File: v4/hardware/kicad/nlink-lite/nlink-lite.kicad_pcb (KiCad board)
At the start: 4 copper layers, 39 x 16 mm, 21 parts, among them J1 USB_MiniB_PLUG_to_calc, J4 PROG_PADS_TC2030, SW1 PWR_SW, U1 ESP32-C3-MINI-1-N4, U3 CP2102N-A02-GQFN24, U4 TLV62569DBV, U5 USBLC6-2SC6

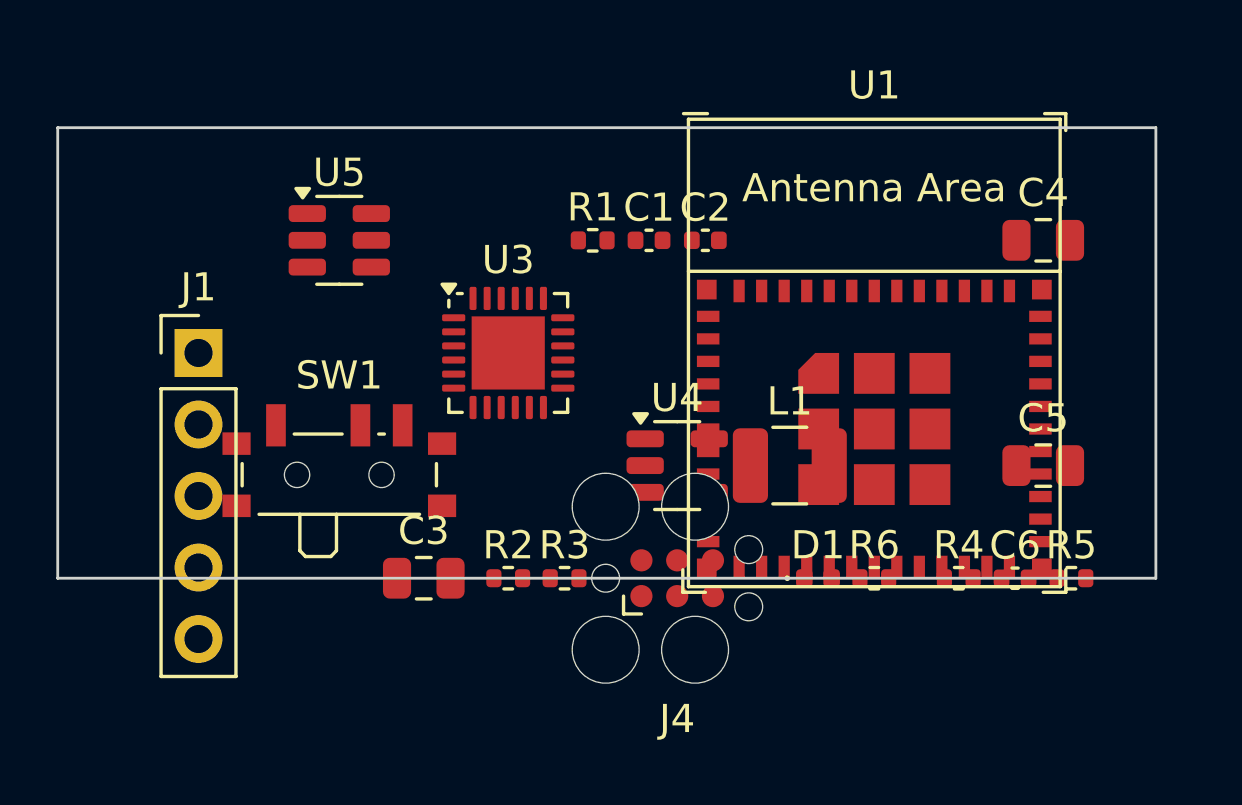
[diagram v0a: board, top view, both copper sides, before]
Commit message: Updated v4 pcb
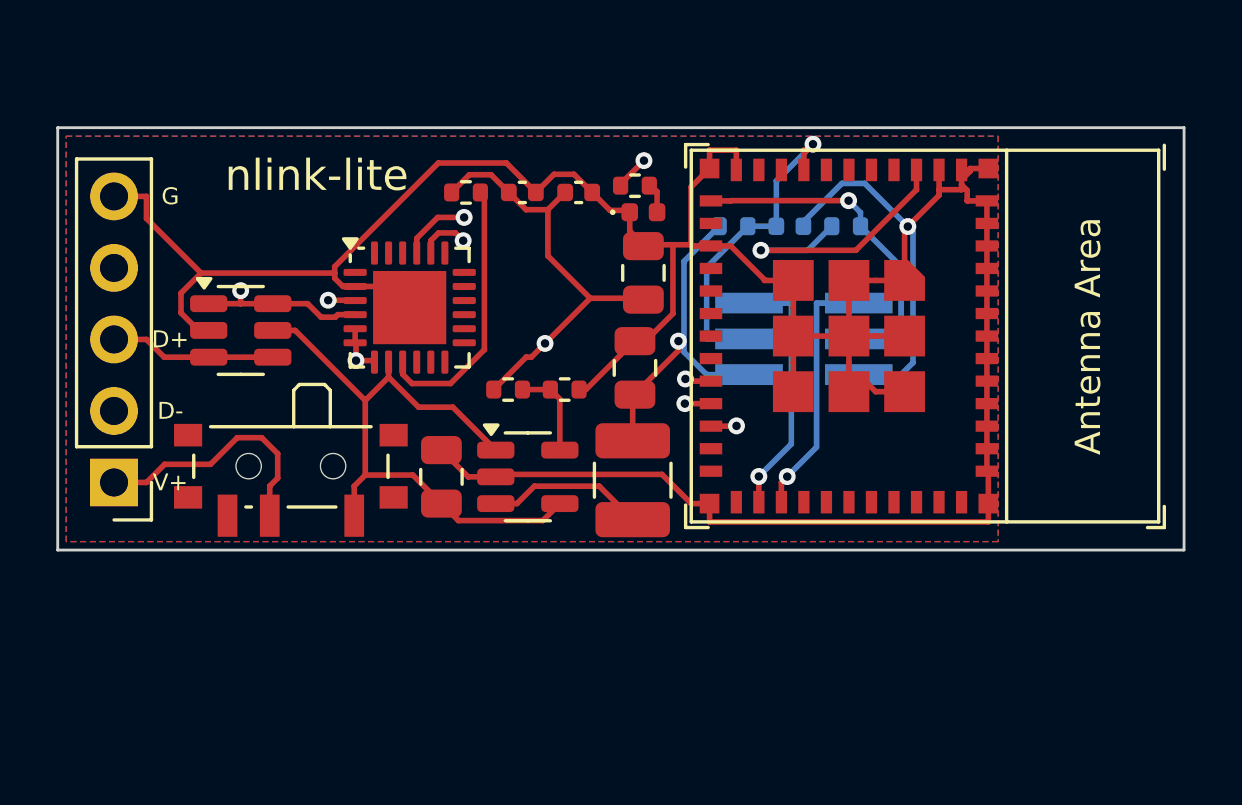
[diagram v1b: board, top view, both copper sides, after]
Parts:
- C6, R4, R5: moved to B.Cu
- J4: value PROG_PADS_TC2030 -> PROG_PADS_2x3_POGO; footprint Connector:Tag-Connect_TC2030-IDC-FP_2x03_P1.27mm_Vertical -> Connector_PinHeader_1.27mm:PinHeader_2x03_P1.27mm_Vertical_SMD; moved to B.Cu
- moved R6 16.3 mm to (70.5, 52.1)
- moved C5 15.8 mm to (70.8, 55.2), turned to 90 degrees
- moved C4 15.2 mm to (70.5, 58.5), turned to 90 degrees
- moved C6 14.8 mm to (76.0, 53.5)
- moved R4 14.8 mm to (74.0, 53.5)
- moved R5 14.8 mm to (78.0, 53.5)
- moved D1 14.4 mm to (70.8, 53.0)
- moved J4 9.62 mm to (76.5, 57.5)
- moved R2 6.70 mm to (66.0, 59.3)
- moved R3 6.70 mm to (68.0, 59.3)
- moved L1 5.60 mm to (70.4, 62.5), turned to 90 degrees
- moved J1 5.49 mm to (52.0, 62.6), turned to 180 degrees
- moved U4 5.32 mm to (66.7, 62.4)
- moved C1 4.81 mm to (66.5, 52.3)
- moved C2 4.81 mm to (68.5, 52.3)
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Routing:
- net GND: track 0.00 -> 117.5 mm, vias 0 -> 1
- net +3V3: track 0.00 -> 55.5 mm, vias 0 -> 4
- net VBUS: track 0.00 -> 23.0 mm
- net CALC_DP: track 0.00 -> 15.0 mm, vias 0 -> 1
- net UART_RX: track 0.00 -> 13.7 mm, vias 0 -> 2
- net UART_TX: track 0.00 -> 13.0 mm, vias 0 -> 2
- net STATUS_LED: track 0.00 -> 12.9 mm, vias 0 -> 2
- net CALC_DM: track 0.00 -> 12.8 mm, vias 0 -> 1
- net IO0: track 0.00 -> 12.1 mm, vias 0 -> 1
- net EN: track 0.00 -> 11.7 mm, vias 0 -> 1
- net CP_RSTn: track 0.00 -> 9.61 mm
- net USB_DP: track 0.00 -> 9.09 mm, vias 0 -> 1
- net USB_DM: track 0.00 -> 9.05 mm, vias 0 -> 1
- net VBUS_IN: track 0.00 -> 9.02 mm
- net SW_NODE: track 0.00 -> 5.61 mm
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- added copper zone on B.Cu, net GND
- added copper zone on F.Cu, net GND
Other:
- board size 39 x 16 mm -> 40 x 15 mm
- board text added: "2:GND 1:3V3"
- board text added: "4:IO0 3:EN"
- board text added: "6:D+ 5:D-"
- board text added: "ANTENNA"
- board text added: "D+"
- board text added: "D-"
- board text added: "G"
- board text added: "PROG"
- board text added: "V+"
- board text added: "nlink-lite"
- board text added: "nlink-lite v4"
- board text removed: "nlink-lite ~38x16 chat-only stealth (placement seed, unrouted)"
